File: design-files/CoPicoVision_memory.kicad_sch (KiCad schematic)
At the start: 4 parts, among them U201 GAL22V10, U202 GAL22V10, U203 AT28C64, U204 AS6C6264

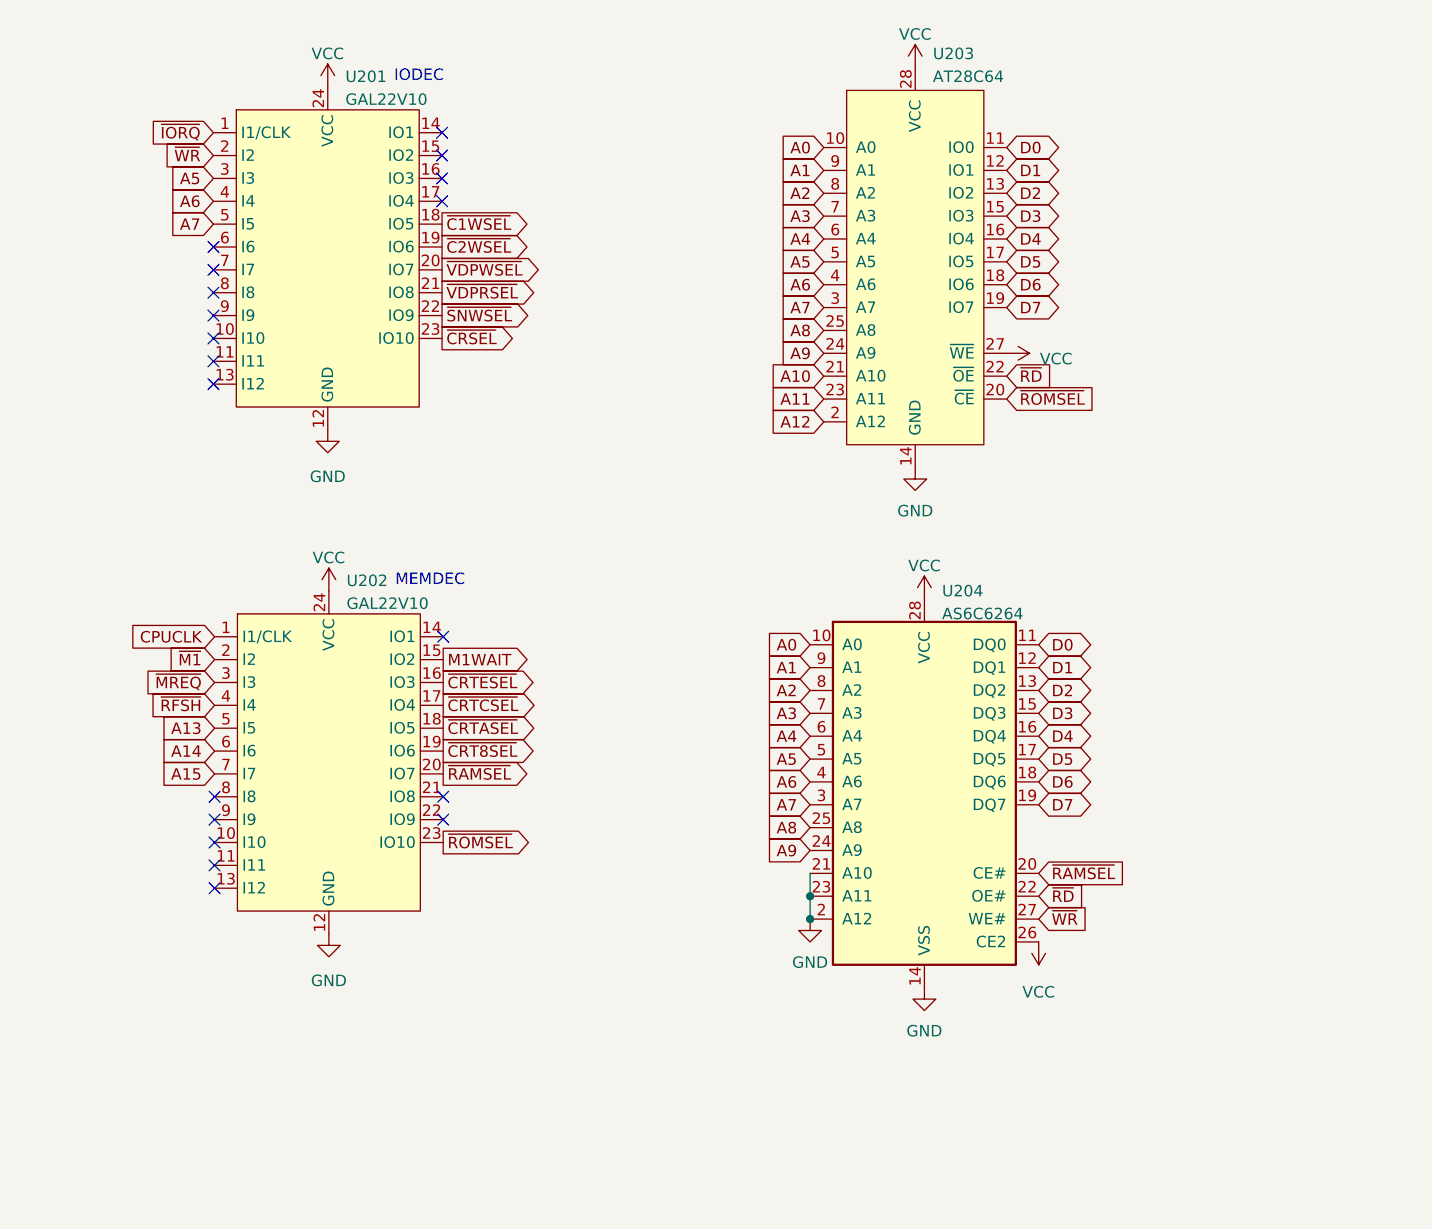
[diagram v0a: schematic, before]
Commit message: Reset and clock.
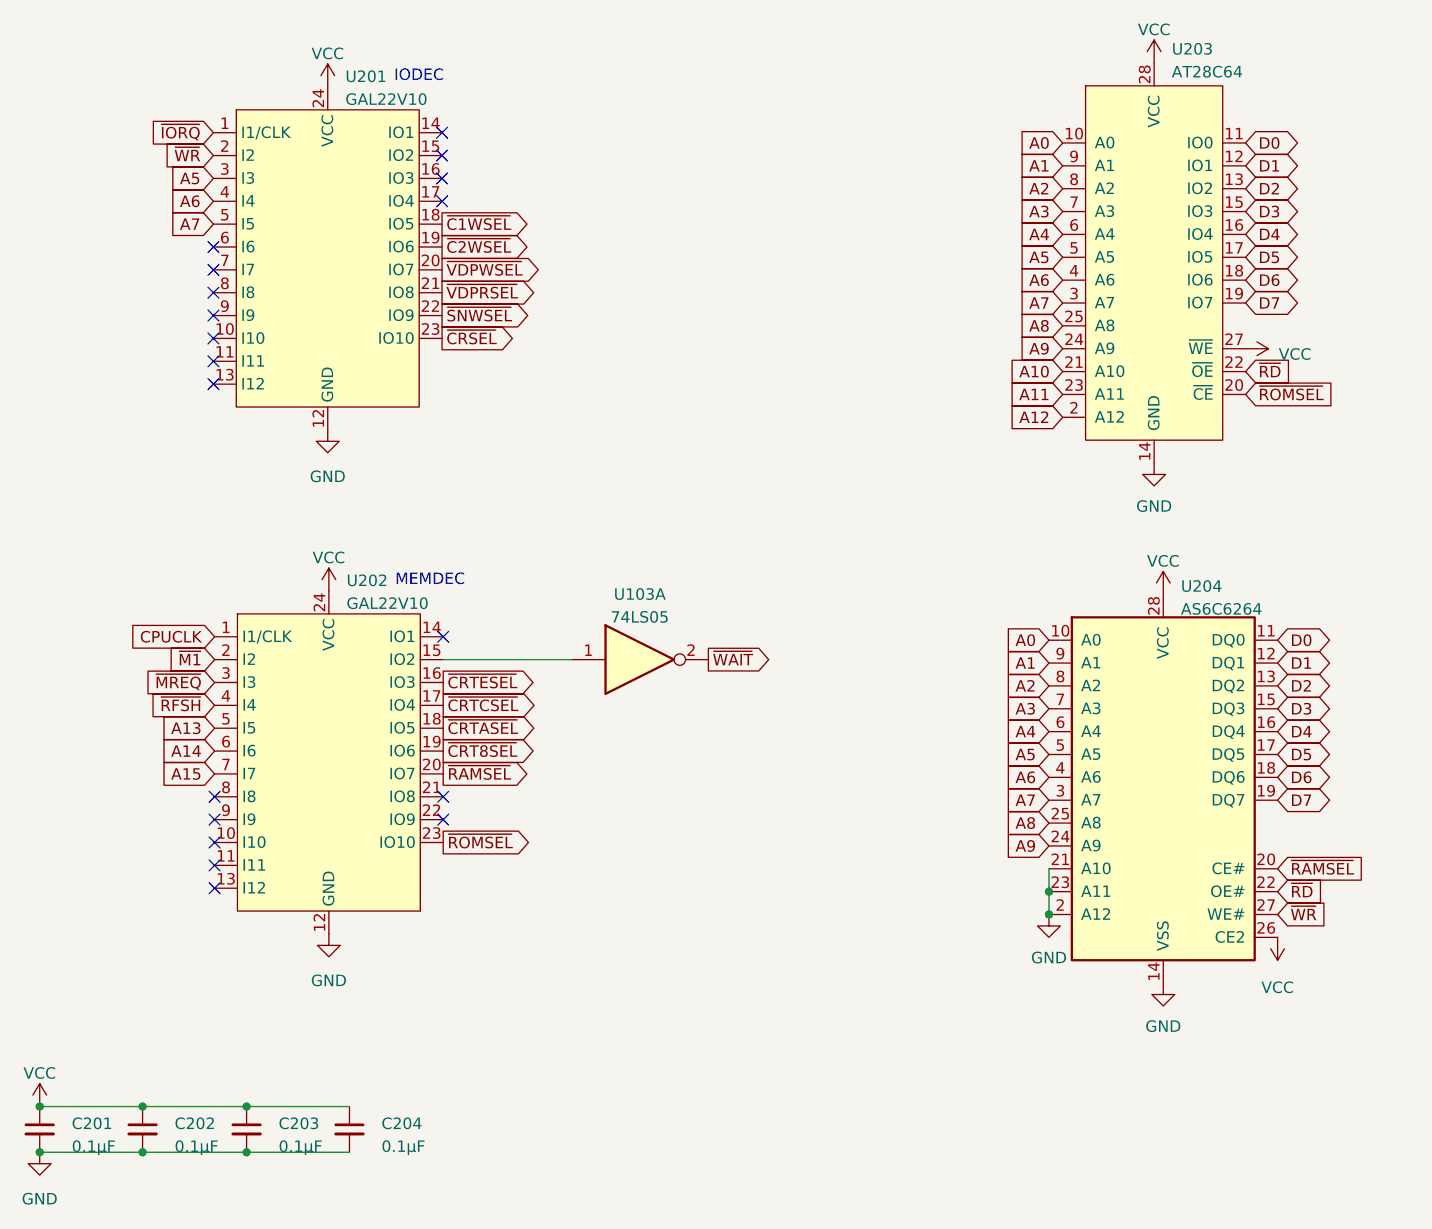
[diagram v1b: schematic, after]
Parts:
- added C201, C202, C203, C204: 0.1µF, symbol Device:C_Small
- added U103: 74LS05, symbol 74xx:74LS05
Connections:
- net GND: now also C201.2, C202.2, C203.2, C204.2
- net VCC: now also C201.1, C202.1, C203.1, C204.1
- net M1WAIT: no longer names the net of U202.15 (IO2)
- net M1WAIT: now also U103.1
- new net ~{WAIT}: U103.2
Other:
- moved on the sheet: U203, U204
